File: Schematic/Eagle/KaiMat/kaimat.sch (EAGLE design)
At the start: 35 parts

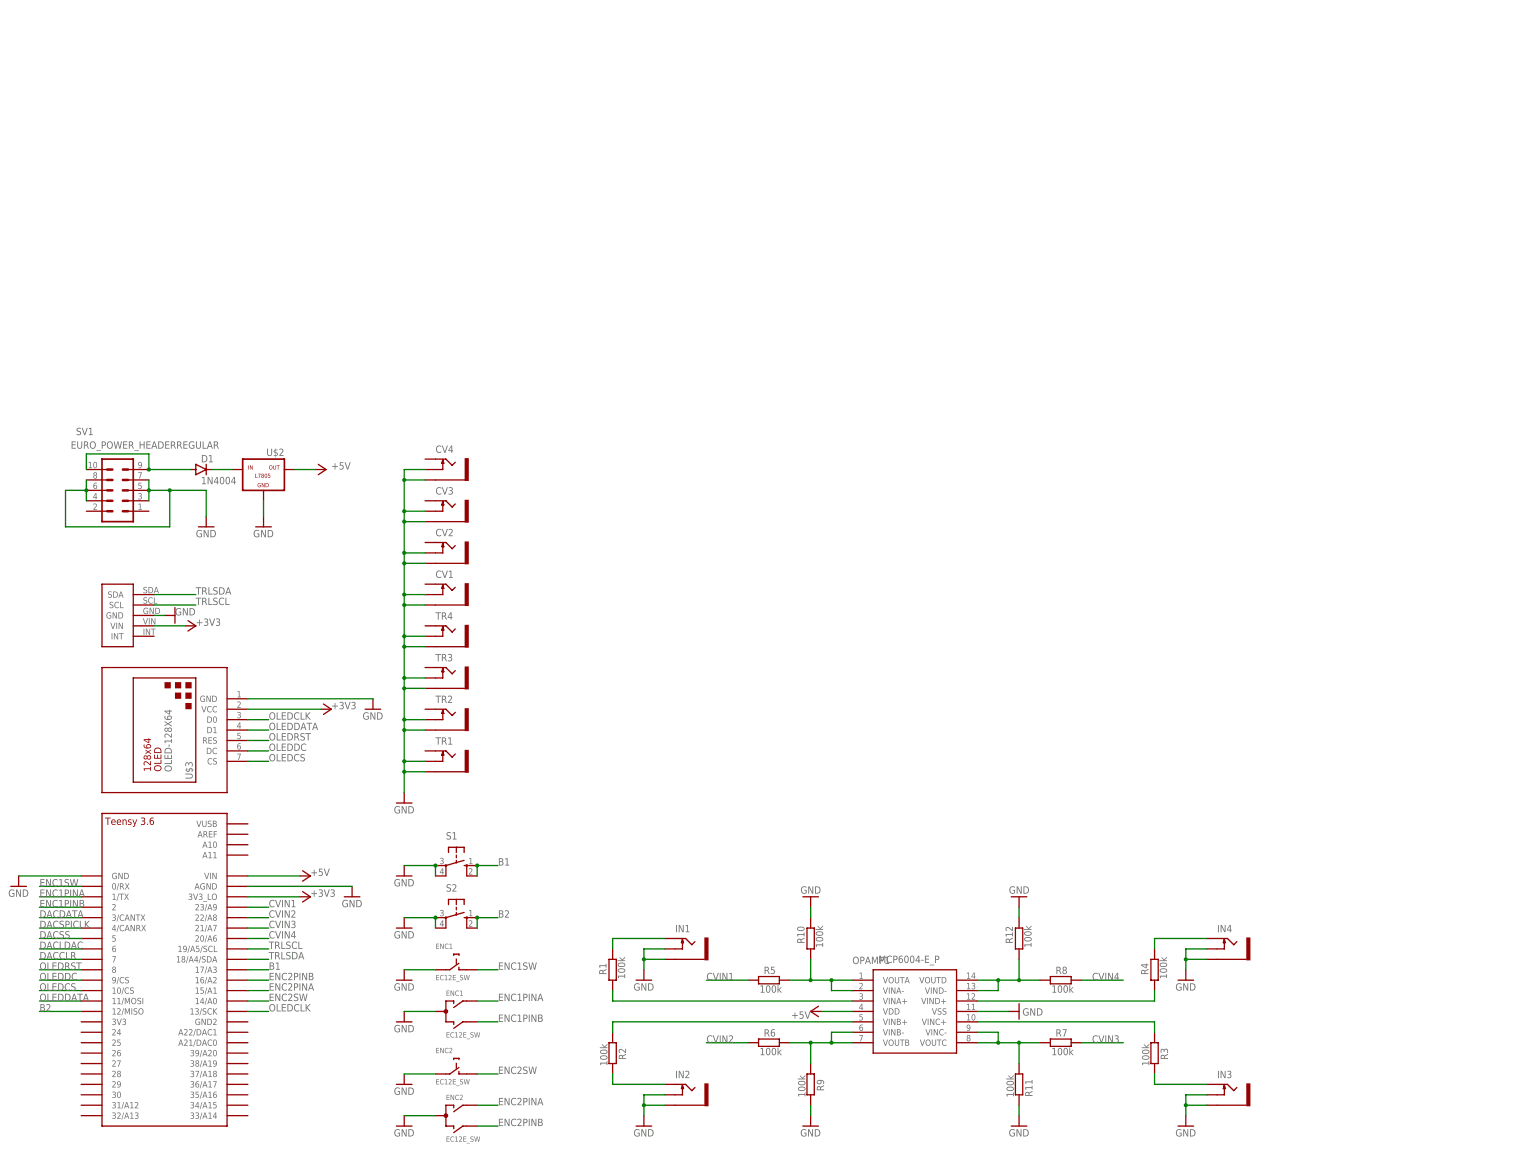
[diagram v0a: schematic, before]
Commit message: improved circuit and pcb£
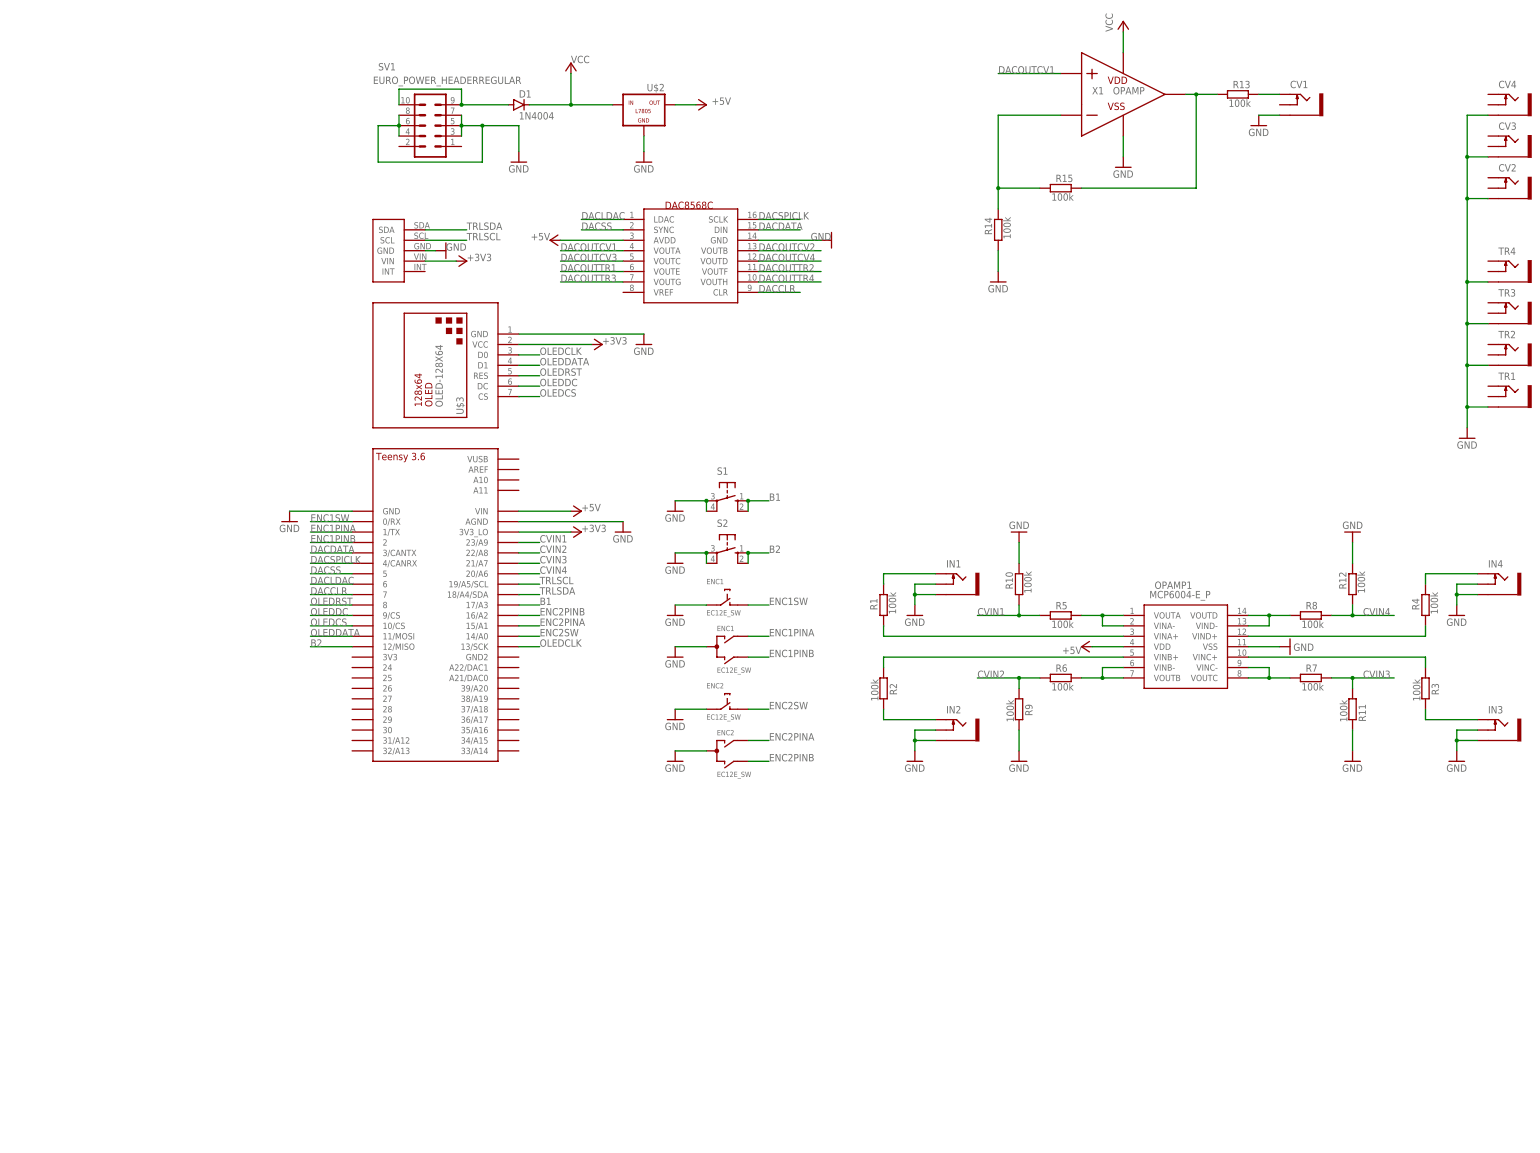
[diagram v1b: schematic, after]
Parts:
- added R13, R14, R15: 100k, MusicThingModular:RESISTOR7MM
- added U$5: DAC8568C, analog-devices-3:DAC8568C
- added X1: OPAMP, ngspice-simulation:OPAMP
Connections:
- removed net N$2: D1.C, U$2.IN
- new net DACOUTCV1: U$5.VOUTA, X1.P
- new net DACOUTCV2: U$5.VOUTB
- new net DACOUTCV3: U$5.VOUTC
- new net DACOUTCV4: U$5.VOUTD
- new net DACOUTTR1: U$5.VOUTE
- new net DACOUTTR2: U$5.VOUTF
- new net DACOUTTR3: U$5.VOUTG
- new net DACOUTTR4: U$5.VOUTH
- new net N$10: R14.2, R15.1, X1.N
- new net N$7: CV1.TIP, R13.2
- new net N$8: R13.1, R15.2, X1.VOUT
- new net VCC: D1.C, U$2.IN, X1.VDD
- net +5V: now also U$5.AVDD
- net CVIN1: now also R10.1
- net CVIN2: now also R9.1
- net CVIN3: now also R11.1
- net CVIN4: now also R12.1
- net DACCLR: now also U$5.CLR
- net DACDATA: now also U$5.DIN
- net DACLDAC: now also U$5.LDAC
- net DACSPICLK: now also U$5.SCLK
- net DACSS: now also U$5.SYNC
- net GND: now also R14.1, U$5.GND, X1.VSS; no longer CV1.SWITCH, CV2.SWITCH, CV3.SWITCH, CV4.SWITCH, TR1.SWITCH, TR2.SWITCH, TR3.SWITCH, TR4.SWITCH
- net N$12: no longer R12.1
- net N$13: no longer R11.1
- net N$18: no longer R10.1
- net N$4: no longer R9.1
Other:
- moved on the sheet: CV1, CV2, CV3, CV4, D1, ENC1, ENC2, IN1, IN2, IN3, IN4, OPAMP1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

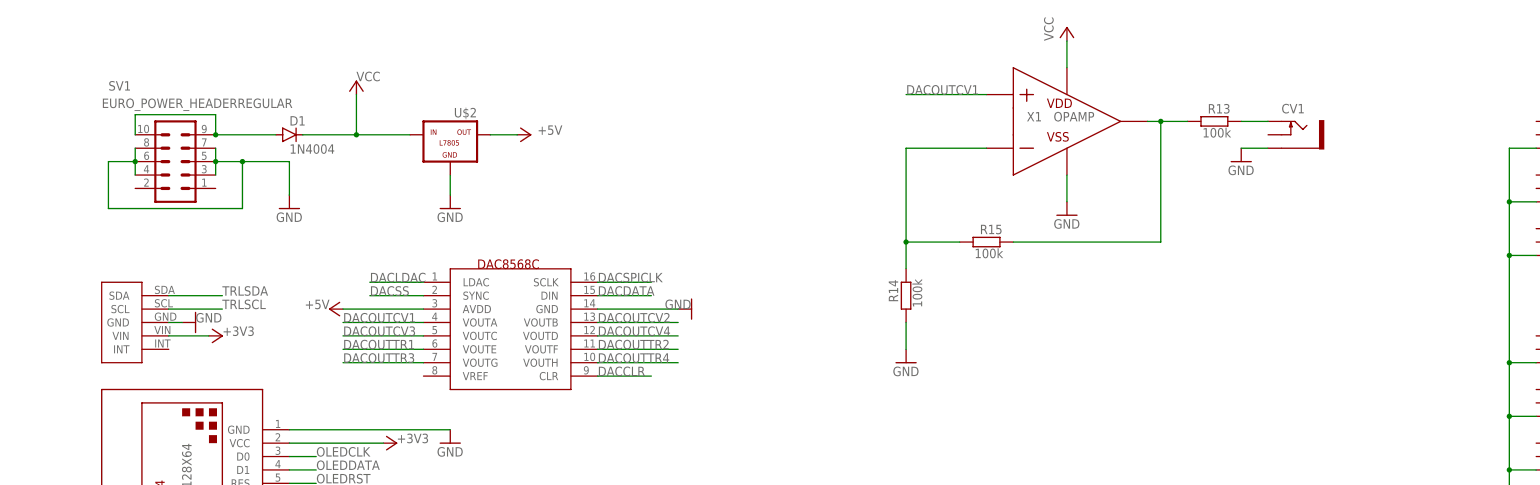
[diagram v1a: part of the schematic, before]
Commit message: updated circuit and pcb
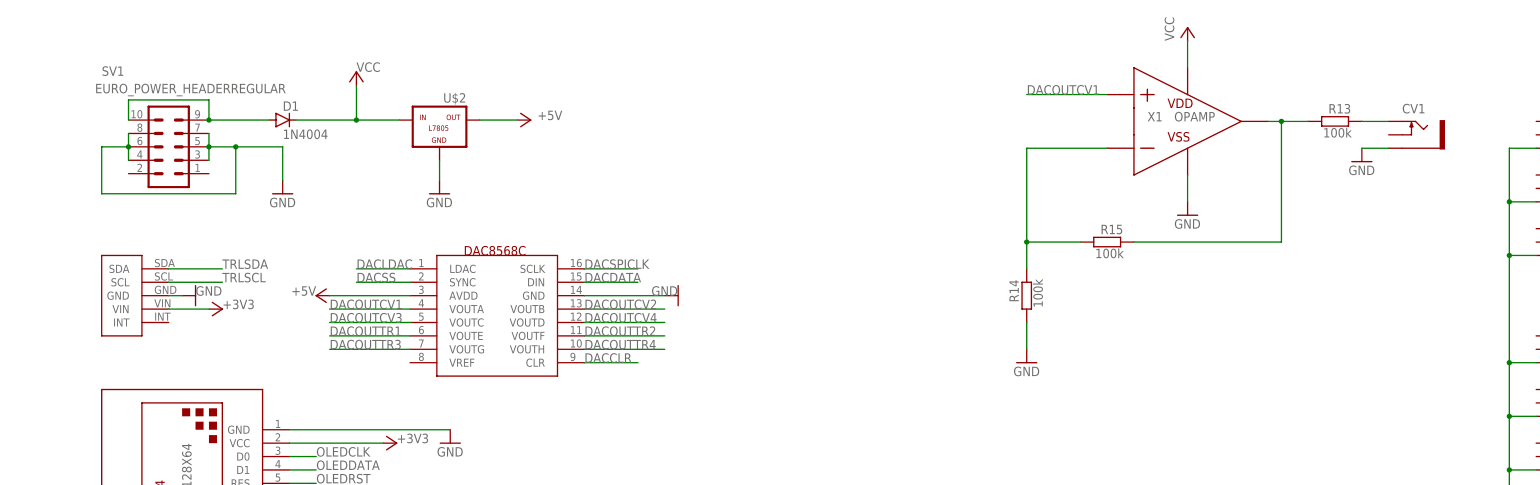
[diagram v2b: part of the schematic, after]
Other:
- moved on the sheet: CV1, D1, R13, R14, R15, SV1, U$2, X1

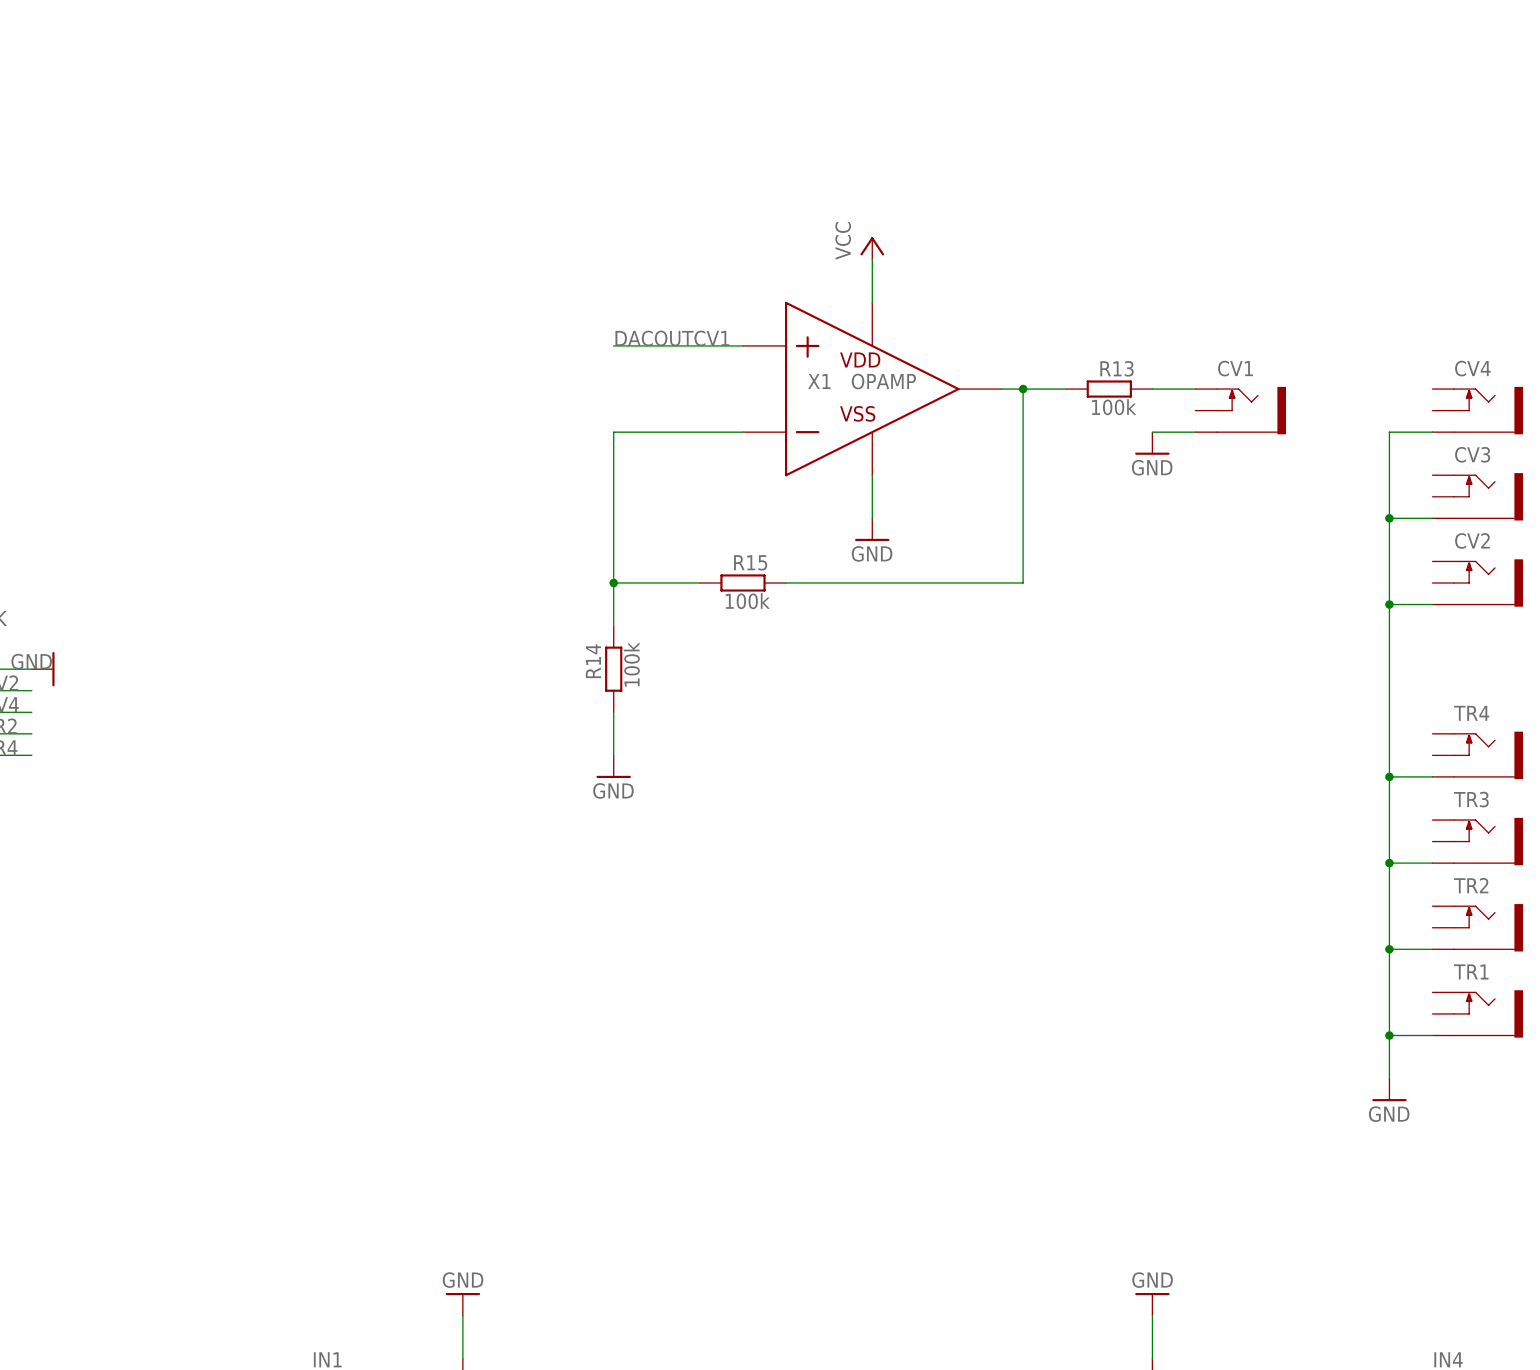
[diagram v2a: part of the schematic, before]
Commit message: updated circuit and pcb
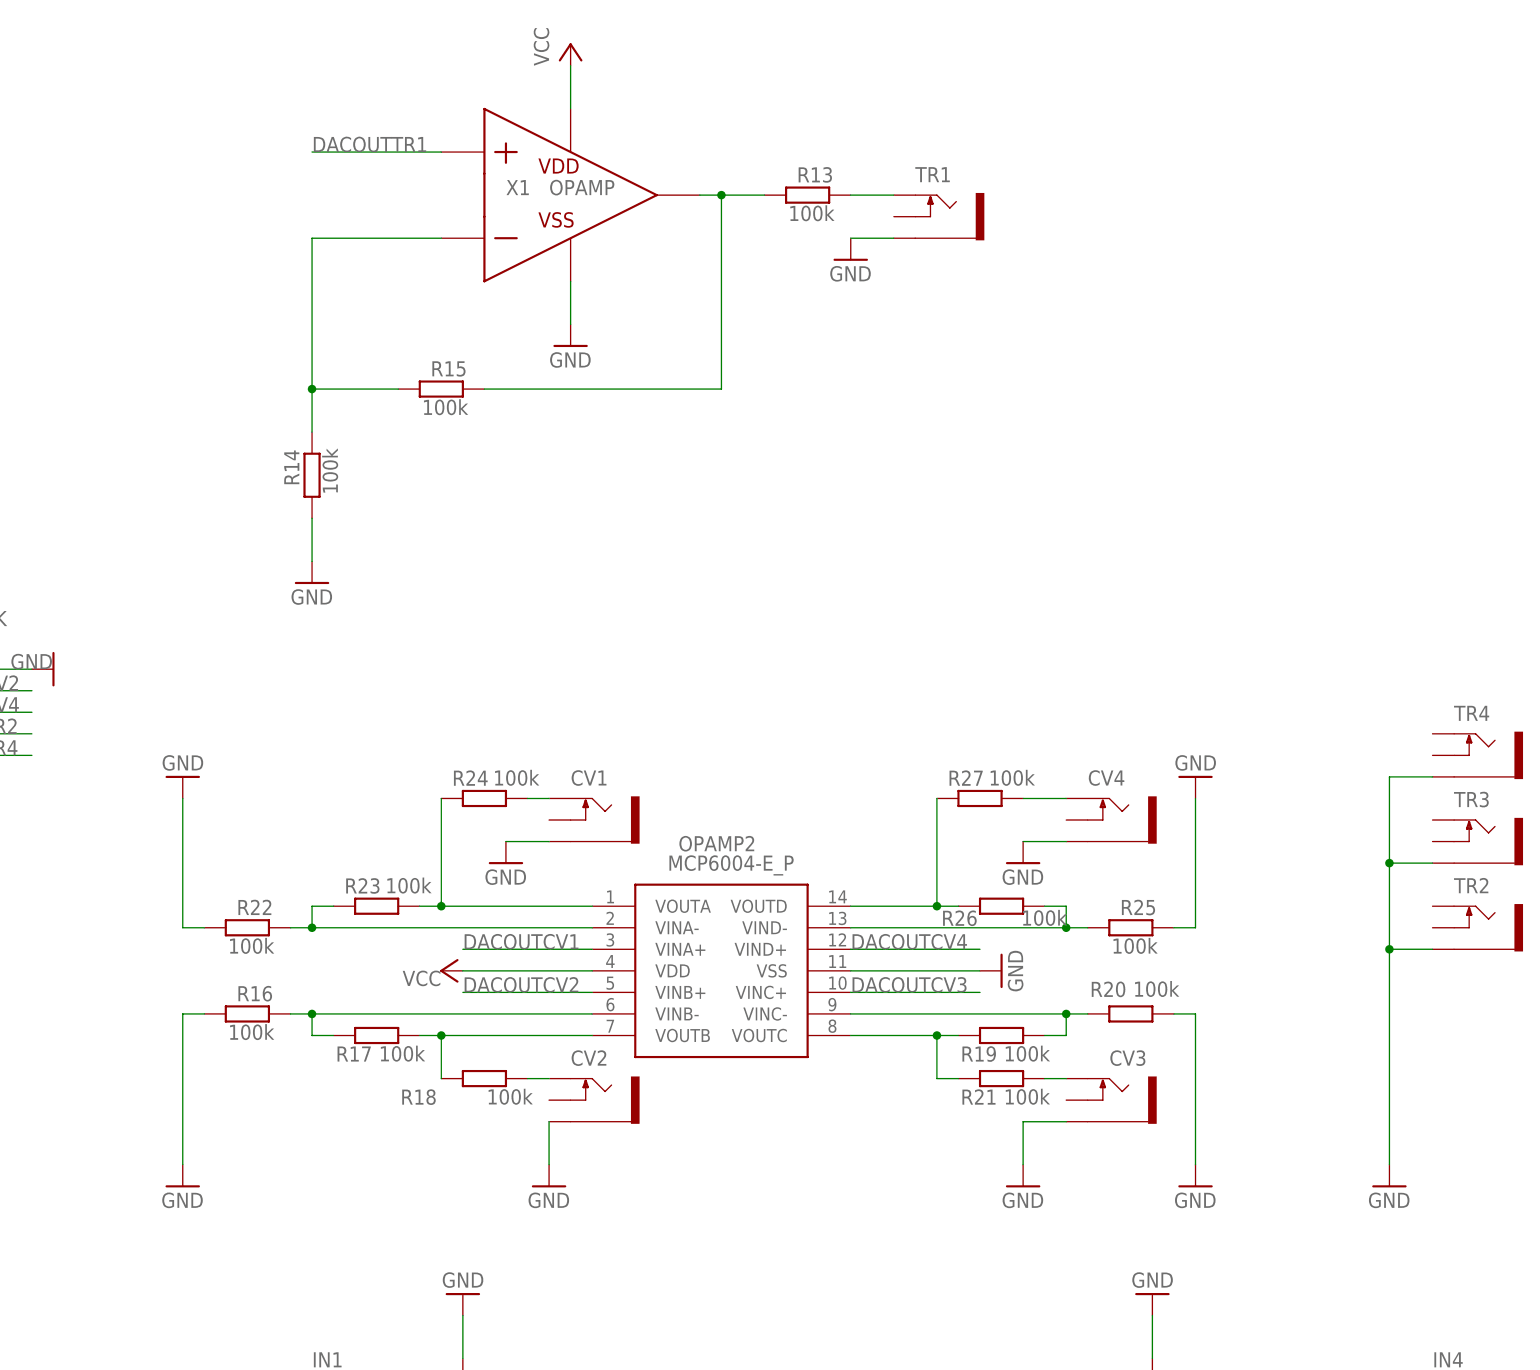
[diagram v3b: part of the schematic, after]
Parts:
- added OPAMP2: MCP6004-E_P, mcp6004-e_p:MCP6004-E_P
- added R16, R17, R18, R19, R20, R21, R22, R23, R24, R25, R26, R27: 100k, MusicThingModular:RESISTOR7MM
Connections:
- new net N$17: OPAMP2.VINB-, R16.2, R17.1
- new net N$19: CV2.TIP, R18.2
- new net N$2: OPAMP2.VOUTB, R17.2, R18.1
- new net N$20: CV3.TIP, R21.2
- new net N$21: OPAMP2.VOUTC, R19.1, R21.1
- new net N$22: OPAMP2.VINC-, R19.2, R20.1
- new net N$23: OPAMP2.VINA-, R22.2, R23.1
- new net N$24: OPAMP2.VOUTA, R23.2, R24.1
- new net N$25: CV1.TIP, R24.2
- new net N$26: OPAMP2.VIND-, R25.1, R26.2
- new net N$27: OPAMP2.VOUTD, R26.1, R27.1
- new net N$28: CV4.TIP, R27.2
- net DACOUTCV1: now also OPAMP2.VINA+; no longer X1.P
- net DACOUTCV2: now also OPAMP2.VINB+
- net DACOUTCV3: now also OPAMP2.VINC+
- net DACOUTCV4: now also OPAMP2.VIND+
- net DACOUTTR1: now also X1.P
- net GND: now also OPAMP2.VSS, R16.1, R20.2, R22.1, R25.2
- net N$7: now also TR1.TIP; no longer CV1.TIP
- net VCC: now also OPAMP2.VDD
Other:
- moved on the sheet: CV1, CV2, CV3, CV4, R13, R14, R15, TR1, X1
